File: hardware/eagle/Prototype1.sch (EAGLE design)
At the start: 26 parts, among them U1 ARDUINO_SHIELDLABEL

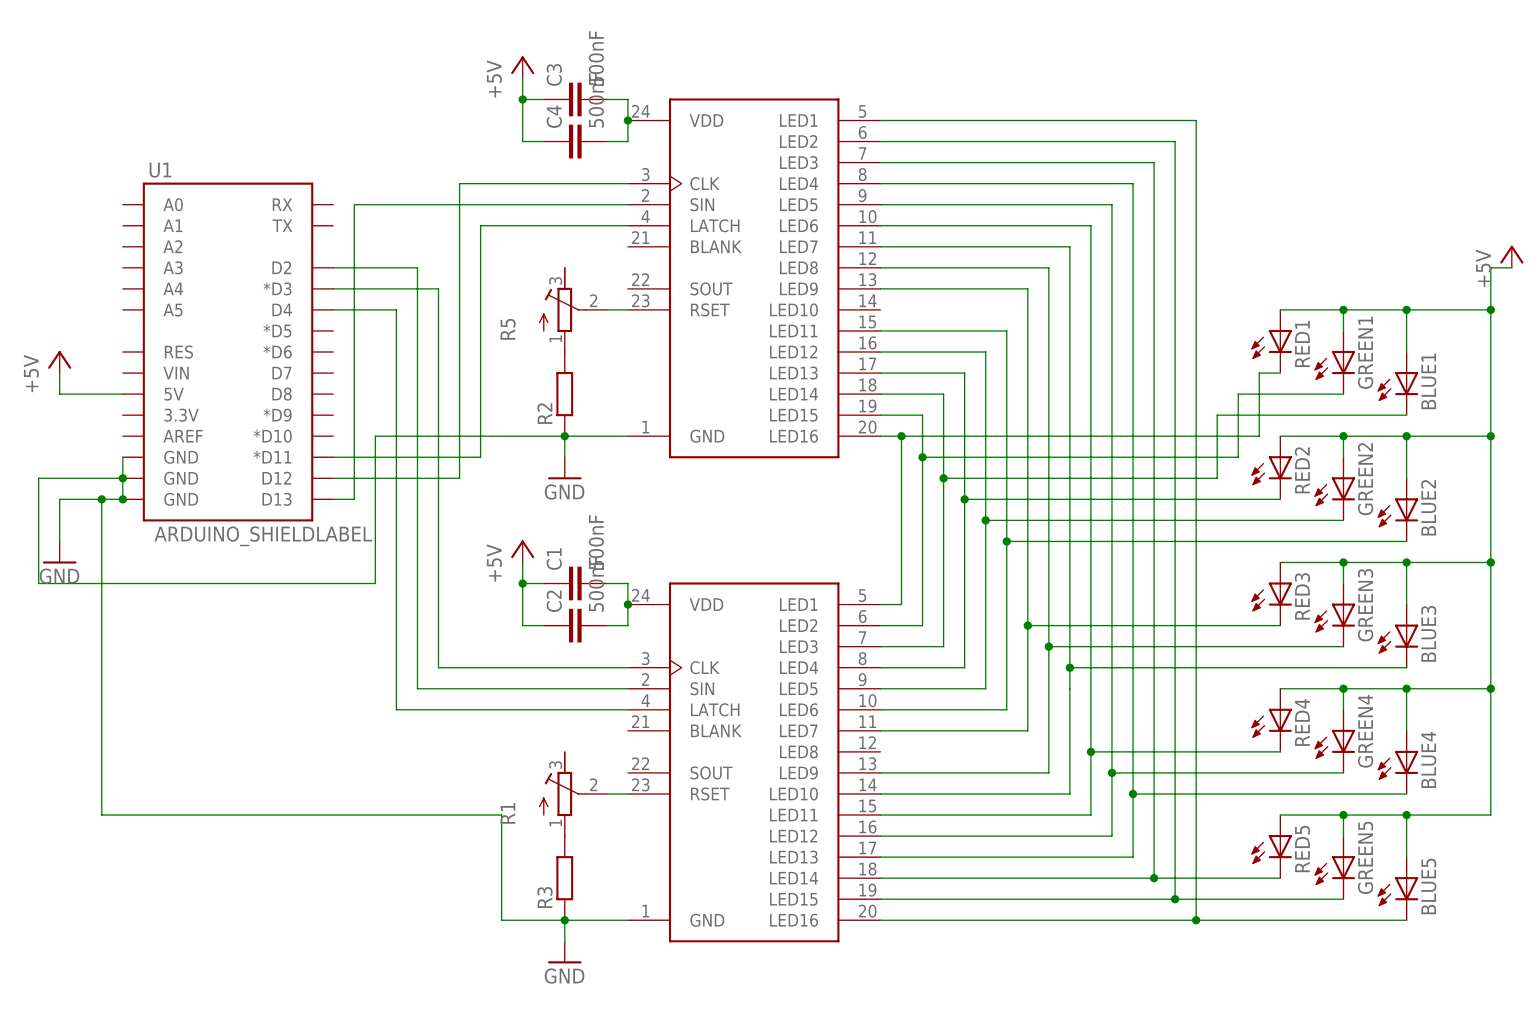
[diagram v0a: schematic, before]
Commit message: finished Prototype1, created gerber
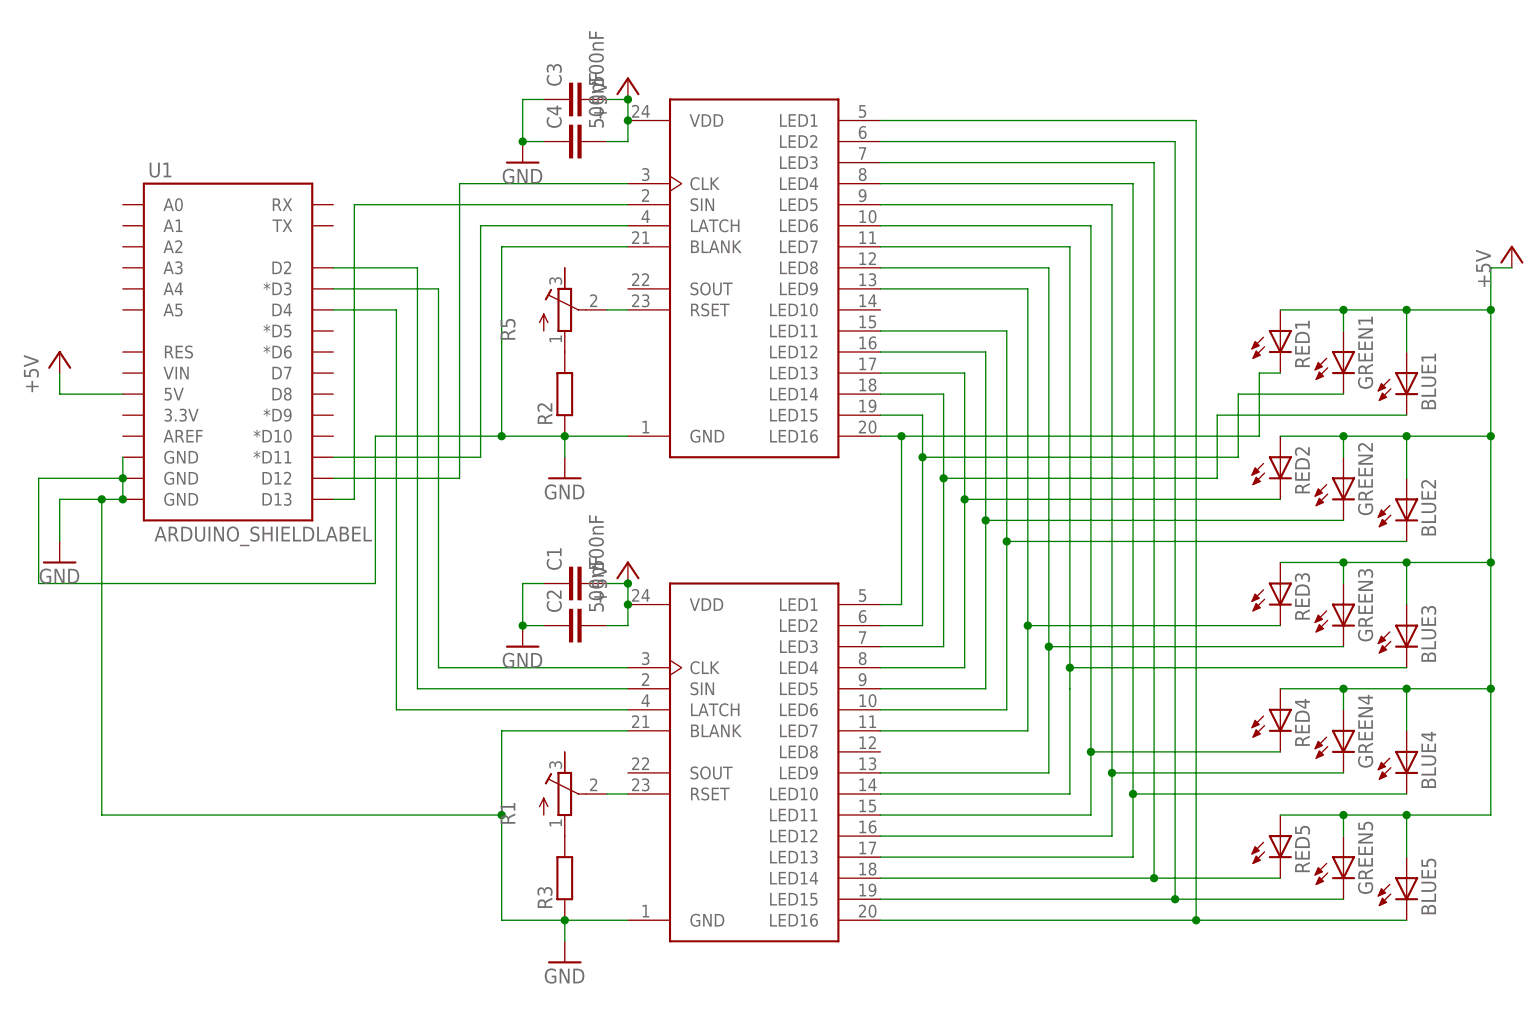
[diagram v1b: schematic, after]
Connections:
- removed net N$1: C1.2, C2.2, U$2.VDD
- removed net N$6: C3.2, C4.2, U$3.VDD
- net +5V: now also C1.2, C2.2, C3.2, C4.2, U$2.VDD, U$3.VDD; no longer C1.1, C2.1, C3.1, C4.1
- net GND: now also C1.1, C2.1, C3.1, C4.1, U$2.BLANK, U$3.BLANK
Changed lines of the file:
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@@
 <part name="GREEN5" library="led" deviceset="LED" device="KA-3528ASYC"/>
 <part name="P+4" library="supply1" deviceset="+5V" device=""/>
+<part name="GND4" library="supply1" deviceset="GND" device=""/>
+<part name="GND5" library="supply1" deviceset="GND" device=""/>
 </parts>
 <sheets>
@@
 <instance part="C2" gate="G$1" x="73.66" y="10.16" rot="R90"/>
 <instance part="U$2" gate="G$1" x="93.98" y="-5.08"/>
-<instance part="P+2" gate="1" x="66.04" y="20.32"/>
+<instance part="P+2" gate="1" x="78.74" y="17.78"/>
 <instance part="R3" gate="G$1" x="71.12" y="-20.32" rot="R90"/>
 <instance part="R1" gate="G$1" x="71.12" y="-10.16"/>
@@
 <instance part="C4" gate="G$1" x="73.66" y="68.58" rot="R90"/>
 <instance part="U$3" gate="G$1" x="93.98" y="53.34"/>
-<instance part="P+3" gate="1" x="66.04" y="78.74"/>
+<instance part="P+3" gate="1" x="78.74" y="76.2"/>
 <instance part="R2" gate="G$1" x="71.12" y="38.1" rot="R90"/>
 <instance part="R5" gate="G$1" x="71.12" y="48.26"/>
@@
 <instance part="GREEN5" gate="G$1" x="165.1" y="-17.78"/>
 <instance part="P+4" gate="1" x="185.42" y="55.88"/>
+<instance part="GND4" gate="1" x="66.04" y="66.04"/>
+<instance part="GND5" gate="1" x="66.04" y="7.62"/>
 </instances>
 <busses>
@@
 <pinref part="U$3" gate="G$1" pin="GND"/>
 <wire x1="78.74" y1="33.02" x2="71.12" y2="33.02" width="0.1524" layer="91"/>
-<wire x1="71.12" y1="33.02" x2="71.12" y2="30.48" width="0.1524" layer="91"/>
 <junction x="71.12" y="33.02"/>
-<wire x1="48.26" y1="33.02" x2="71.12" y2="33.02" width="0.1524" layer="91"/>
+<wire x1="48.26" y1="33.02" x2="63.5" y2="33.02" width="0.1524" layer="91"/>
 <wire x1="48.26" y1="33.02" x2="48.26" y2="15.24" width="0.1524" layer="91"/>
 <wire x1="48.26" y1="15.24" x2="7.62" y2="15.24" width="0.1524" layer="91"/>
@@
 <junction x="17.78" y="25.4"/>
 <junction x="15.24" y="25.4"/>
+<pinref part="U$3" gate="G$1" pin="BLANK"/>
+<wire x1="78.74" y1="55.88" x2="63.5" y2="55.88" width="0.1524" layer="91"/>
+<wire x1="63.5" y1="55.88" x2="63.5" y2="33.02" width="0.1524" layer="91"/>
+<wire x1="63.5" y1="33.02" x2="71.12" y2="33.02" width="0.1524" layer="91"/>
+<wire x1="71.12" y1="33.02" x2="71.12" y2="30.48" width="0.1524" layer="91"/>
+<junction x="63.5" y="33.02"/>
+<pinref part="U$2" gate="G$1" pin="BLANK"/>
+<wire x1="78.74" y1="-2.54" x2="63.5" y2="-2.54" width="0.1524" layer="91"/>
+<wire x1="63.5" y1="-2.54" x2="63.5" y2="-12.7" width="0.1524" layer="91"/>
+<junction x="63.5" y="-12.7"/>
+</segment>
+<segment>
+<pinref part="C3" gate="G$1" pin="1"/>
+<wire x1="68.58" y1="73.66" x2="66.04" y2="73.66" width="0.1524" layer="91"/>
+<pinref part="C4" gate="G$1" pin="1"/>
+<wire x1="68.58" y1="68.58" x2="66.04" y2="68.58" width="0.1524" layer="91"/>
+<wire x1="66.04" y1="68.58" x2="66.04" y2="73.66" width="0.1524" layer="91"/>
+<pinref part="GND4" gate="1" pin="GND"/>
+<junction x="66.04" y="68.58"/>
+</segment>
+<segment>
+<pinref part="C1" gate="G$1" pin="1"/>
+<wire x1="68.58" y1="15.24" x2="66.04" y2="15.24" width="0.1524" layer="91"/>
+<pinref part="C2" gate="G$1" pin="1"/>
+<wire x1="68.58" y1="10.16" x2="66.04" y2="10.16" width="0.1524" layer="91"/>
+<wire x1="66.04" y1="10.16" x2="66.04" y2="15.24" width="0.1524" layer="91"/>
+<pinref part="GND5" gate="1" pin="GND"/>
+<junction x="66.04" y="10.16"/>
 </segment>
 </net>
@@
 <pinref part="U1" gate="G$1" pin="5V"/>
 <wire x1="10.16" y1="38.1" x2="17.78" y2="38.1" width="0.1524" layer="91"/>
-</segment>
-<segment>
-<pinref part="C1" gate="G$1" pin="1"/>
-<pinref part="P+2" gate="1" pin="+5V"/>
-<wire x1="68.58" y1="15.24" x2="66.04" y2="15.24" width="0.1524" layer="91"/>
-<wire x1="66.04" y1="15.24" x2="66.04" y2="17.78" width="0.1524" layer="91"/>
-<pinref part="C2" gate="G$1" pin="1"/>
-<wire x1="68.58" y1="10.16" x2="66.04" y2="10.16" width="0.1524" layer="91"/>
-<wire x1="66.04" y1="10.16" x2="66.04" y2="15.24" width="0.1524" layer="91"/>
-<junction x="66.04" y="15.24"/>
-</segment>
-<segment>
-<pinref part="C3" gate="G$1" pin="1"/>
-<pinref part="P+3" gate="1" pin="+5V"/>
-<wire x1="68.58" y1="73.66" x2="66.04" y2="73.66" width="0.1524" layer="91"/>
-<wire x1="66.04" y1="73.66" x2="66.04" y2="76.2" width="0.1524" layer="91"/>
-<pinref part="C4" gate="G$1" pin="1"/>
-<wire x1="68.58" y1="68.58" x2="66.04" y2="68.58" width="0.1524" layer="91"/>
-<wire x1="66.04" y1="68.58" x2="66.04" y2="73.66" width="0.1524" layer="91"/>
-<junction x="66.04" y="73.66"/>
 </segment>
 <segment>
@@
 <junction x="165.1" y="48.26"/>
 </segment>
-</net>
-<net name="N$2" class="0">
-<segment>
-<pinref part="R1" gate="G$1" pin="A"/>
-<pinref part="R3" gate="G$1" pin="2"/>
-</segment>
-</net>
-<net name="N$4" class="0">
-<segment>
-<pinref part="U$2" gate="G$1" pin="RSET"/>
-<pinref part="R1" gate="G$1" pin="S"/>
-<wire x1="78.74" y1="-10.16" x2="76.2" y2="-10.16" width="0.1524" layer="91"/>
-</segment>
-</net>
-<net name="N$1" class="0">
+<segment>
+<pinref part="U$3" gate="G$1" pin="VDD"/>
+<wire x1="78.74" y1="71.12" x2="78.74" y2="68.58" width="0.1524" layer="91"/>
+<pinref part="C4" gate="G$1" pin="2"/>
+<wire x1="78.74" y1="68.58" x2="76.2" y2="68.58" width="0.1524" layer="91"/>
+<wire x1="78.74" y1="71.12" x2="78.74" y2="73.66" width="0.1524" layer="91"/>
+<pinref part="C3" gate="G$1" pin="2"/>
+<wire x1="78.74" y1="73.66" x2="76.2" y2="73.66" width="0.1524" layer="91"/>
+<junction x="78.74" y="71.12"/>
+<pinref part="P+3" gate="1" pin="+5V"/>
+<junction x="78.74" y="73.66"/>
+</segment>
 <segment>
 <pinref part="U$2" gate="G$1" pin="VDD"/>
@@
 <wire x1="78.74" y1="15.24" x2="76.2" y2="15.24" width="0.1524" layer="91"/>
 <junction x="78.74" y="12.7"/>
+<pinref part="P+2" gate="1" pin="+5V"/>
+<junction x="78.74" y="15.24"/>
+</segment>
+</net>
+<net name="N$2" class="0">
+<segment>
+<pinref part="R1" gate="G$1" pin="A"/>
+<pinref part="R3" gate="G$1" pin="2"/>
+</segment>
+</net>
+<net name="N$4" class="0">
+<segment>
+<pinref part="U$2" gate="G$1" pin="RSET"/>
+<pinref part="R1" gate="G$1" pin="S"/>
+<wire x1="78.74" y1="-10.16" x2="76.2" y2="-10.16" width="0.1524" layer="91"/>
 </segment>
 </net>
@@
 </segment>
 </net>
-<net name="N$6" class="0">
-<segment>
-<pinref part="U$3" gate="G$1" pin="VDD"/>
-<wire x1="78.74" y1="71.12" x2="78.74" y2="68.58" width="0.1524" layer="91"/>
-<pinref part="C4" gate="G$1" pin="2"/>
-<wire x1="78.74" y1="68.58" x2="76.2" y2="68.58" width="0.1524" layer="91"/>
-<wire x1="78.74" y1="71.12" x2="78.74" y2="73.66" width="0.1524" layer="91"/>
-<pinref part="C3" gate="G$1" pin="2"/>
-<wire x1="78.74" y1="73.66" x2="76.2" y2="73.66" width="0.1524" layer="91"/>
-<junction x="78.74" y="71.12"/>
-</segment>
-</net>
